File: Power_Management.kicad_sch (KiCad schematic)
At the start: 17 parts, among them IC2 OpAmp_NE5532D, J13 I2S_OR_LJ_OUT, J8 JST_XH_2.54_Plug_5V+, Q2 MOSFET_SI2333DDS-T1-BE3

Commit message: Update
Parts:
- removed C21, C24: 47u, Capacitor_SMD:C_0805_2012Metric, symbol Device:C_Polarized
- removed C22, C23: 10n_X7R, Capacitor_SMD:C_0805_2012Metric, symbol Device:C
- removed FB1: BLM21PG601SN1D_0805, Capacitor_SMD:C_0805_2012Metric, symbol Device:FerriteBead
- removed J13: I2S_OR_LJ_OUT, Connector_PinHeader_2.54mm:PinHeader_1x03_P2.54mm_Vertical, symbol Connector_Generic:Conn_01x03
- removed J8: JST_XH_2.54_Plug_5V+, Personal_Project:Connector_Power2pin_SHDRRA2W80P0X250_1X2_740X1150X610P, symbol Personal_Projects:Connector_Power2pin_JST_XH_2.54_Plug
- removed LDO2: LDO_TLV75733PDBVR, Personal_Project:LDO_SOT95P280X145-5N, symbol Personal_Projects:LDO_TLV75733PDBVR
- removed Q2: MOSFET_SI2333DDS-T1-BE3, Personal_Project:MOSFET_ SI2333DDS_SOT_DS-T1-BE3_VIS, symbol Personal_Projects:MOSFET_SI2333DDS-T1-BE3
- removed R7: 100k, Resistor_SMD:R_0805_2012Metric, symbol Device:R
- removed S1: Switch_WS-SLSU SMT Mini Slide, Personal_Project:Switch_WS-SLSU SMT Mini Slide, symbol Personal_Projects:Switch_WS-SLSU SMT Mini Slide
- removed Z2, Z3: Diode_BZX84C6V2-7-F, Personal_Project:Diode_BZX84C6V2_SOT96P240X110-3N, symbol Personal_Projects:Diode_BZX84C6V2-7-F
- added C19: 1u, Capacitor_SMD:C_0805_2012Metric, symbol Device:C
- added C20: 2u2, Capacitor_SMD:C_0805_2012Metric, symbol Device:C
- added C25, C27: 10u, Capacitor_SMD:C_0805_2012Metric, symbol Device:C
- added C30: 470n, Capacitor_SMD:C_0805_2012Metric, symbol Device:C
- added C33, C36: 47u, Capacitor_SMD:C_0805_2012Metric, symbol Device:C_Polarized
- added C34, C35: 10n_X7R, Capacitor_SMD:C_0805_2012Metric, symbol Device:C
- added D1: SMAJ6.0A, Personal_Project:DO-214AC-2, symbol Personal_Projects:DIODE_SMAJ6.0A
- added FB2: BLM21PG601SN1D_0805, Capacitor_SMD:C_0805_2012Metric, symbol Device:FerriteBead
- added J1: JST_XH_2.54_Plug_5V+, Personal_Project:Connector_Power2pin_SHDRRA2W80P0X250_1X2_740X1150X610P, symbol Personal_Projects:Connector_Power2pin_JST_XH_2.54_Plug
- added J3: I2S_OR_LJ_OUT, Connector_PinHeader_2.54mm:PinHeader_1x03_P2.54mm_Vertical, symbol Connector_Generic:Conn_01x03
- added LDO1: LDO_LDLN050PUR, Package_DFN_QFN:DFN-8-1EP_3x3mm_P0.65mm_EP1.7x2.05mm, symbol Personal_Projects:LDO_LDLN050PUR
- added LDO2: LDO_LDLN050PU33R, Package_DFN_QFN:DFN-8-1EP_3x3mm_P0.65mm_EP1.7x2.05mm, symbol Personal_Projects:LDO_LDLN050PUR
- added LDO3: LDO_LD39200PU33R, Package_DFN_QFN:DFN-6-1EP_3x3mm_P0.95mm_EP1.7x2.6mm, symbol Personal_Projects:LDO_LD39200PU33R
- added Q1: MOSFET_SI2333DDS-T1-BE3, Personal_Project:MOSFET_ SI2333DDS_SOT_DS-T1-BE3_VIS, symbol Personal_Projects:MOSFET_SI2333DDS-T1-BE3
- added R10, R6: 31k6, Resistor_SMD:R_0805_2012Metric, symbol Device:R
- added R11, R14, R9: 10k, Resistor_SMD:R_0805_2012Metric, symbol Device:R
- added R12: 100k, Resistor_SMD:R_0805_2012Metric, symbol Device:R
- added R13: 90k, Resistor_SMD:R_0805_2012Metric, symbol Device:R
- added S2: Switch_WS-SLSU SMT Mini Slide, Personal_Project:Switch_WS-SLSU SMT Mini Slide, symbol Personal_Projects:Switch_WS-SLSU SMT Mini Slide
- added Z1: Diode_BZX84C6V2-7-F, Personal_Project:Diode_BZX84C6V2_SOT96P240X110-3N, symbol Personal_Projects:Diode_BZX84C6V2-7-F
- C18: value 1u -> 2u2
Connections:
- net +3.3V: now also C27.1, C30.1, LDO2.1 (OUT), LDO3.1 (OUT), R10.1, R13.2
- net +5VA: now also C35.1, C36.1, FB2.2; no longer C1.1
- net EXT_POWER_5V+: now also J1.2 (POWER+), Q1.3 (D)
- net EXT_POWER_5V+_PP: now also J3.3 (Pin_3), Q1.2 (S), Z1.3 (K)
- net GND: now also C19.2, C20.2, C25.2, C27.2, C33.2, C34.2, C35.2, C36.2, D1.2 (A), J1.1 (POWER-), LDO1.4 (GND_1), LDO1.9 (GND_2), LDO2.4 (GND_1), LDO2.9 (GND_2), LDO3.3 (GND), LDO3.7 (EPAD), R11.2, R12.2, R14.1, R9.2
- net MOSFET_GATE_5V: now also Q1.1 (G), R12.1, Z1.1 (A)
- net USB_VBUS_5V: now also J3.1 (Pin_1)
- new net: LDO1.3 (FB), R6.2, R9.1
- new net: J3.2 (Pin_2), S2.2
- new net: C30.2, LDO3.2 (ADJ/SENSE), R13.1, R14.2
- new net: LDO2.3 (FB), R10.2, R11.1
- new net EN: LDO3.5 (EN)
- new net OUT_LD39200DPUR: C20.1, C25.1, C33.1, C34.1, FB2.1, LDO1.1 (OUT), LDO3.6 (IN), R6.1
- new net PG: LDO3.4 (PG)
- new net VIN_LDLN050PUR: C1.1, C19.1, D1.1 (K), LDO1.5 (EN), LDO1.8 (IN), LDO2.5 (EN), LDO2.8 (IN), S2.1
- no-connect marks 5 -> 11
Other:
- note added: "Protects the MAX 6V VIN"
- note added: "To LDO_LD39200PU33R 3V3 LDO"
- note added: "VIN from 1.25 V to 6.0 V"
- note added: "VIN: 2.7 V to 6.5 V"
- note added: "VOUT​=1.208⋅(1+31600/10000)≈5.0253 V"
- note removed: "If shutdown capability is not required, connect EN to IN."
- moved on the sheet: C17, IC2

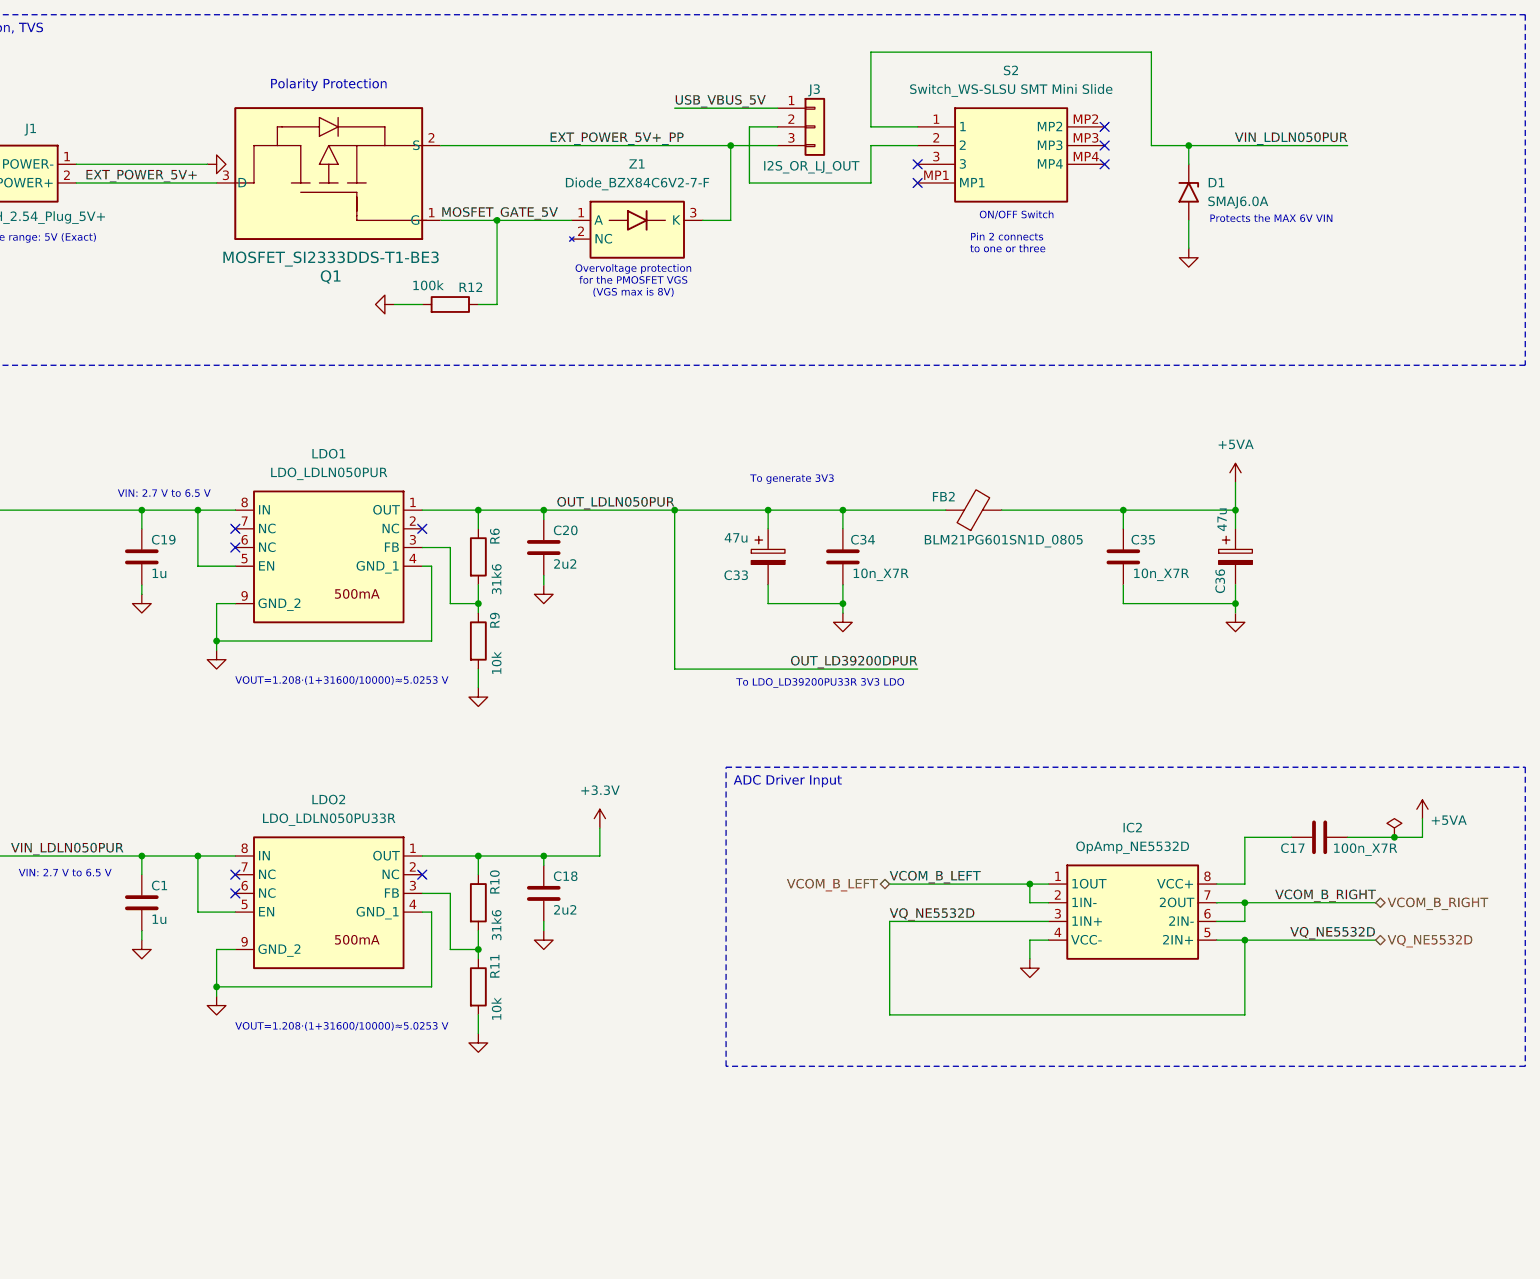
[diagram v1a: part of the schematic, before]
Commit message: Update
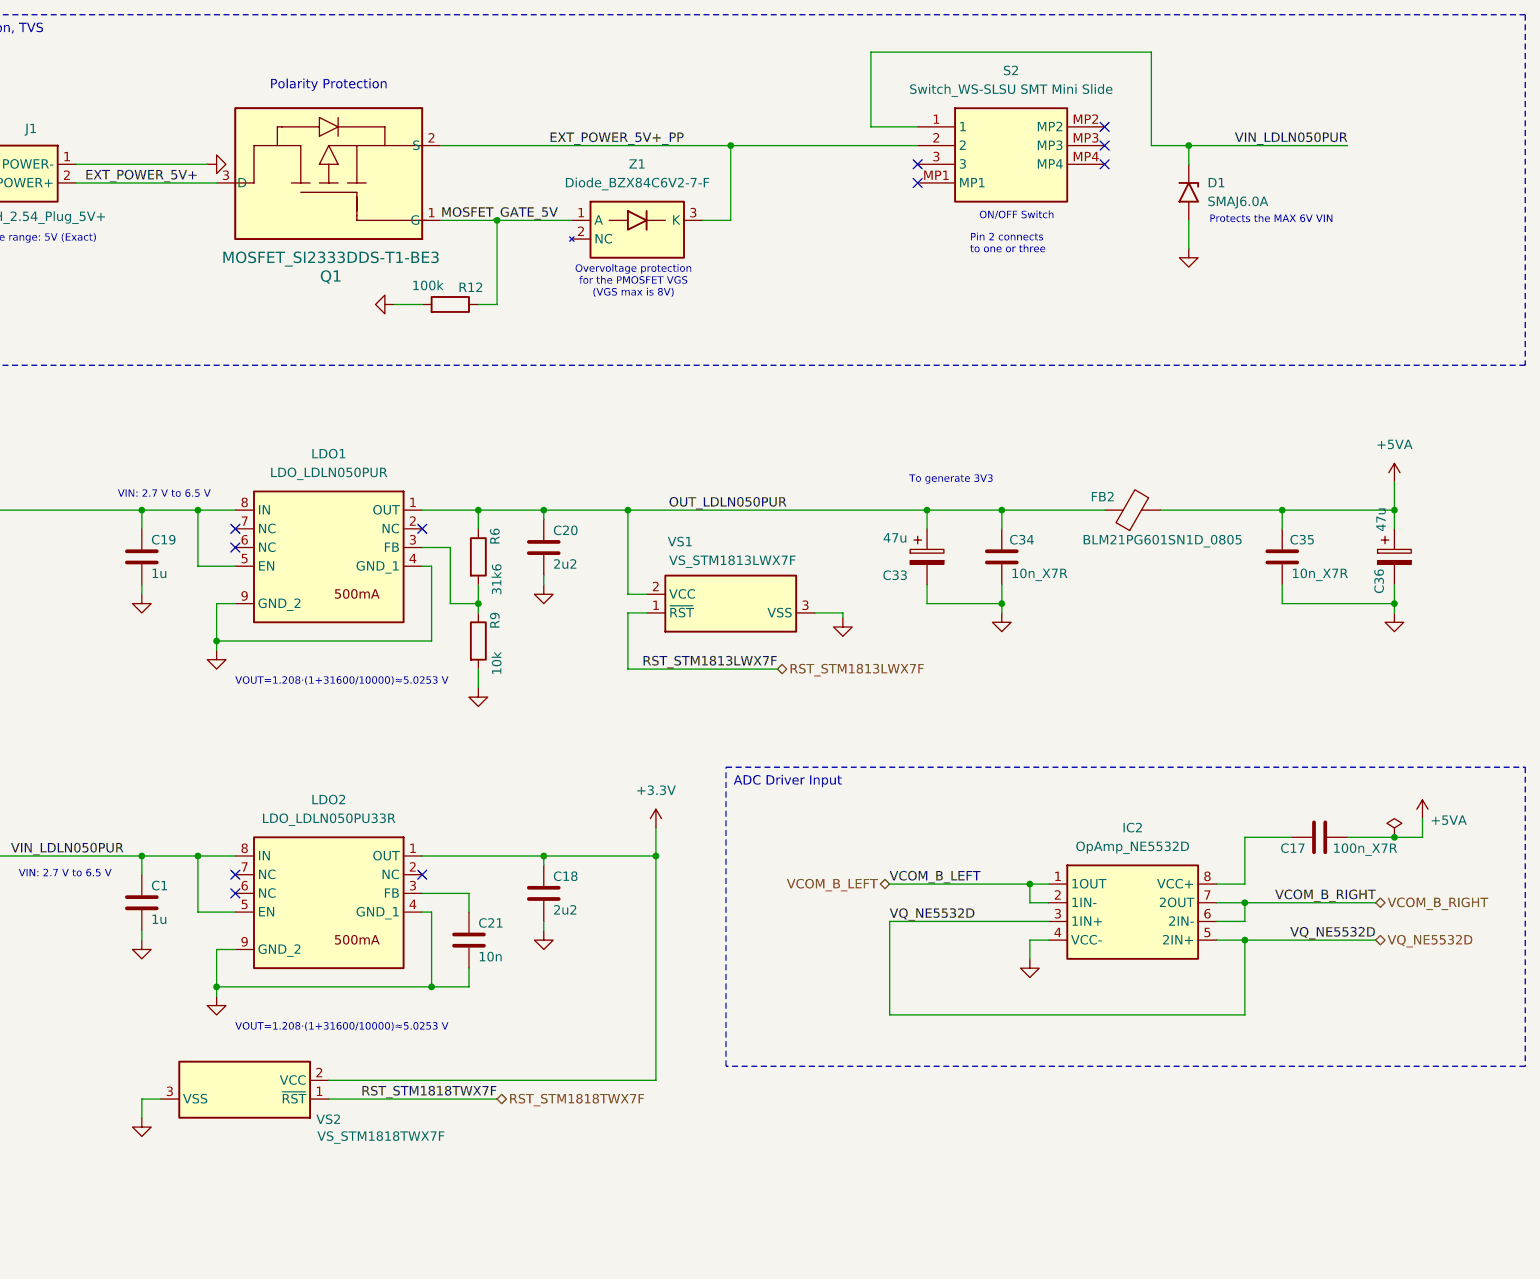
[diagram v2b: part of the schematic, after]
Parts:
- removed J3: I2S_OR_LJ_OUT, Connector_PinHeader_2.54mm:PinHeader_1x03_P2.54mm_Vertical, symbol Connector_Generic:Conn_01x03
- removed R10: 31k6, Resistor_SMD:R_0805_2012Metric, symbol Device:R
- removed R11: 10k, Resistor_SMD:R_0805_2012Metric, symbol Device:R
- added C21: 10n, Capacitor_SMD:C_0805_2012Metric, symbol Device:C
- added VS1: VS_STM1813LWX7F, Personal_Project:SOT-23-3_SOT103P237X112-3N, symbol Personal_Projects:VS_STM1813LWX7F
- added VS2: VS_STM1818TWX7F, Personal_Project:SOT-23-3_SOT103P237X112-3N, symbol Personal_Projects:VS_STM1813LWX7F
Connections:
- net +3.3V: now also VS2.2 (VCC)
- net EXT_POWER_5V+_PP: now also S2.2
- net GND: now also C21.2, VS1.3 (VSS), VS2.3 (VSS)
- net OUT_LD39200DPUR: no longer C20.1, C33.1, C34.1, FB2.1, LDO1.1 (OUT), R6.1
- net at LDO2.3 (FB): now also C21.1
- new net OUT_LDLN050PUR: C20.1, C33.1, C34.1, FB2.1, LDO1.1 (OUT), R6.1, VS1.2 (VCC)
- new net RST_STM1813LWX7F: VS1.1 (~{RST})
- new net RST_STM1818TWX7F: VS2.1 (~{RST})
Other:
- note removed: "To LDO_LD39200PU33R 3V3 LDO"
- moved on the sheet: C33, C34, C35, C36, FB2
